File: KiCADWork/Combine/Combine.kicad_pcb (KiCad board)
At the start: 2 copper layers, 100 x 100 mm, 147 parts, among them J1 USB_C_Receptacle, J3 USB_C_Receptacle, J4 Conn_01x10_Socket, J4 Screw_Terminal_01x01, J5 Screw_Terminal_01x02, J6 USB_C_Receptacle, J7 Screw_Terminal_01x01, J8 Screw_Terminal_01x02, P1 USB_C_Plug, P2 USB_C_Plug, SW1 TK-6580B-1, SW2 SW_DIP_x01, SW3 TK-6580B-1, U1 AMS1117-3.3, U2 BQ24073RGT, U3 TPS61023DRLR, U4 SIP32509DT-T1-GE3, U5 USB2422T-I/MJ, U6 SIP32509DT-T1-GE3, U7 MCP73831T-2ACI/OT, U8 XB6096I2SV, U9 NRF52833-QDAA-R7, Y1 X322524MOB4SI, Y2 X161032768KLD2SI, Y3 XL7EL89CKI-111YLC-32M

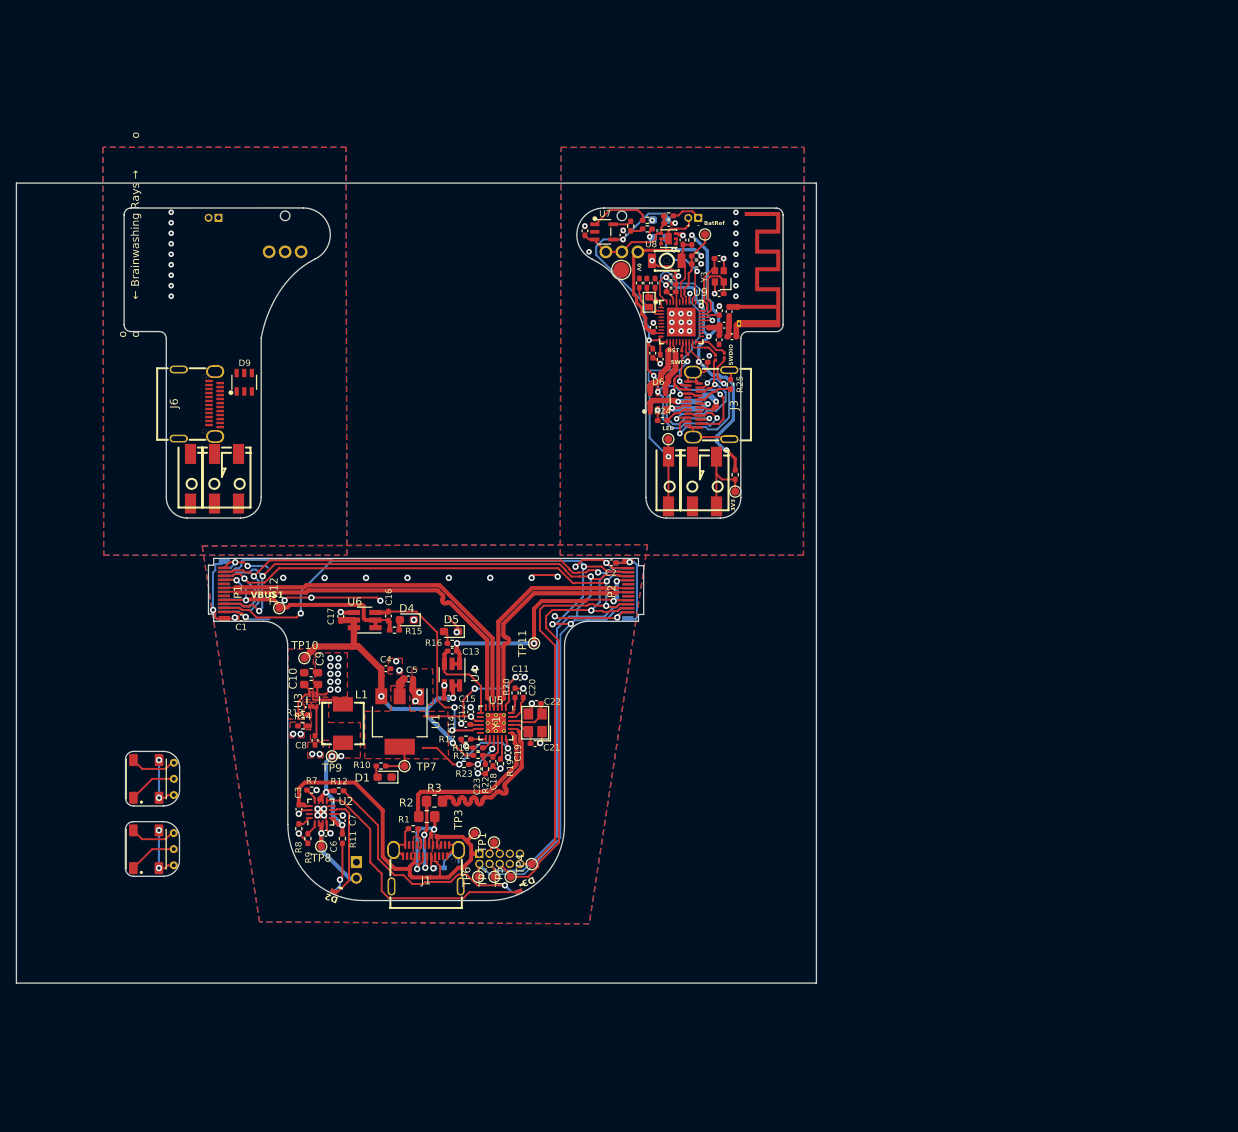
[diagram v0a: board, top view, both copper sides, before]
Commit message: Schem rev 1 pt1
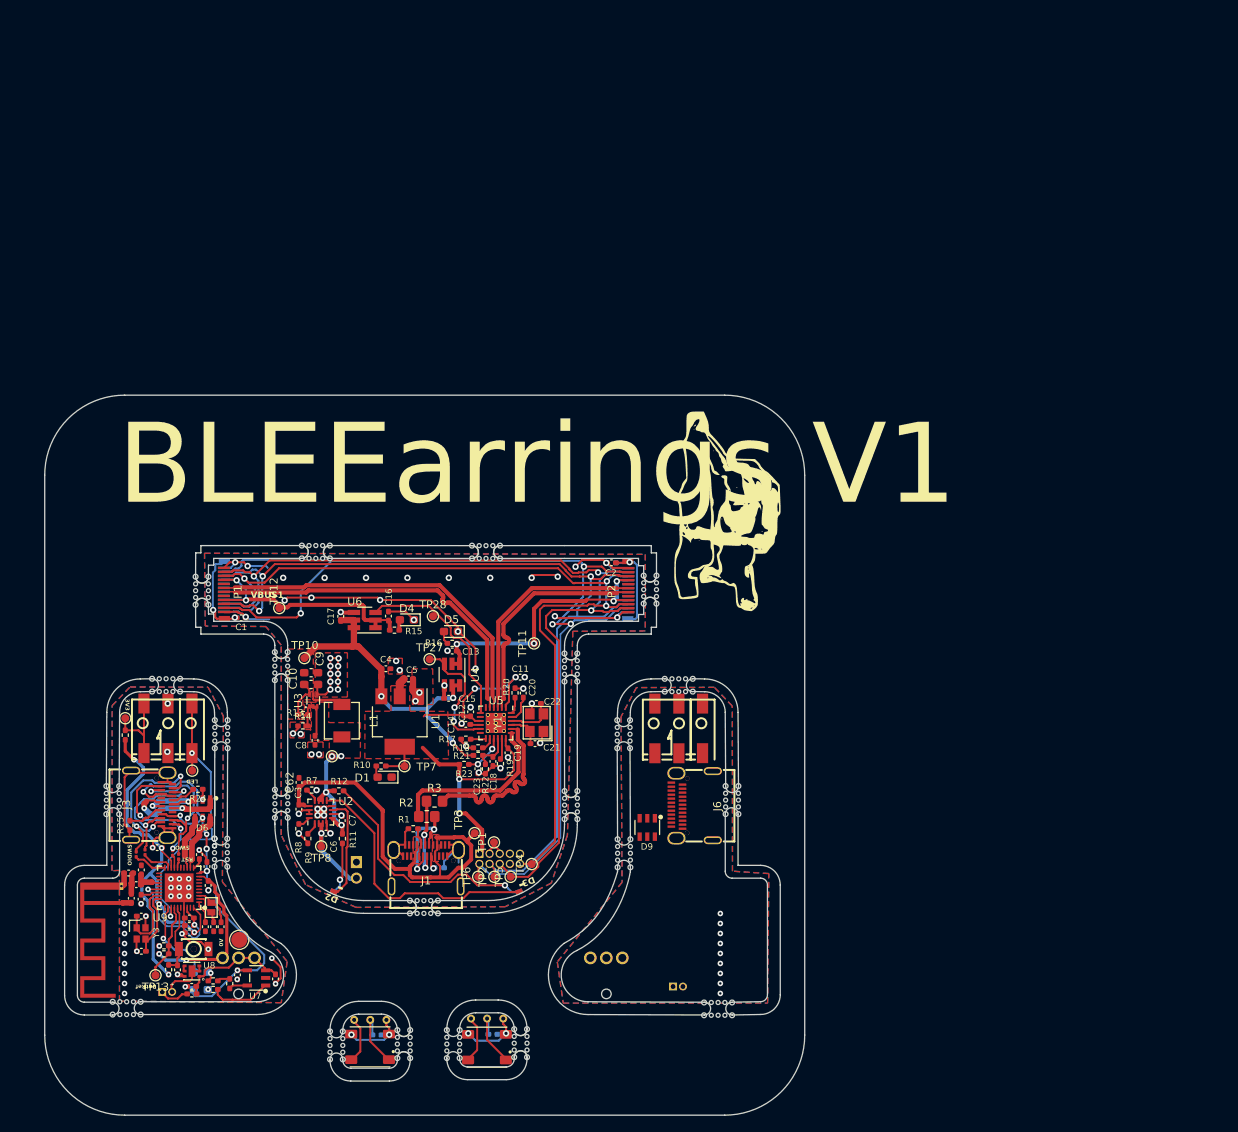
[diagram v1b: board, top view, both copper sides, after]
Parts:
- removed the TP9 at (133.5, 115.2)
- added ?: , , F.Cu at (118.8, 125.5)
- added ?: , , F.Cu at (118.8, 126.4)
- added C62: 10u, Capacitor_SMD:C_0402_1005Metric_Pad0.74x0.62mm_HandSolder, F.Cu at (129.4, 118.5)
- added C63: 100n, Capacitor_SMD:C_0402_1005Metric_Pad0.74x0.62mm_HandSolder, B.Cu at (153.6, 150.0)
- added C64: 100n, Capacitor_SMD:C_0402_1005Metric_Pad0.74x0.62mm_HandSolder, B.Cu at (139.1, 150.0)
- added G***: LOGO, CustomPads:OT2, F.Cu at (182.7, 84.4)
- added REF**: mouse-bit-1.6mm-slot, Panelization:mouse-bit-1.6mm-slot, F.Cu at (127.2, 121.1)
- added REF**: mouse-bit-1.6mm-slot, Panelization:mouse-bit-1.6mm-slot, F.Cu at (163.4, 121.3)
- added REF**: mouse-bit-1.6mm-slot, Panelization:mouse-bit-1.6mm-slot, F.Cu at (157.1, 151.1)
- added REF**: mouse-bit-1.6mm-slot, Panelization:mouse-bit-1.6mm-slot, B.Cu at (181.8, 146.8)
- added REF**: mouse-bit-1.6mm-slot, Panelization:mouse-bit-1.6mm-slot, B.Cu at (112.8, 106.3)
- added REF**: mouse-bit-1.6mm-slot, Panelization:mouse-bit-1.6mm-slot, B.Cu at (134.1, 151.3)
- added REF**: mouse-bit-1.6mm-slot, Panelization:mouse-bit-1.6mm-slot, B.Cu at (107.8, 146.7)
- added REF**: mouse-bit-1.6mm-slot, Panelization:mouse-bit-1.6mm-slot, B.Cu at (106.1, 120.7)
- added REF**: mouse-bit-1.6mm-slot, Panelization:mouse-bit-1.6mm-slot, B.Cu at (183.5, 120.7)
- added REF**: mouse-bit-1.6mm-slot, Panelization:mouse-bit-1.6mm-slot, B.Cu at (119.7, 112.4)
- added REF**: mouse-bit-1.6mm-slot, Panelization:mouse-bit-1.6mm-slot, B.Cu at (119.6, 127.3)
- added REF**: mouse-bit-1.6mm-slot, Panelization:mouse-bit-1.6mm-slot, F.Cu at (127.2, 103.9)
- added REF**: mouse-bit-1.6mm-slot, Panelization:mouse-bit-1.6mm-slot, B.Cu at (148.7, 151.2)
- added REF**: mouse-bit-1.6mm-slot, Panelization:mouse-bit-1.6mm-slot, B.Cu at (170.0, 127.3)
- added REF**: mouse-bit-1.6mm-slot, Panelization:mouse-bit-1.6mm-slot, B.Cu at (170.0, 112.4)
- added REF**: mouse-bit-1.6mm-slot, Panelization:mouse-bit-1.6mm-slot, B.Cu at (176.8, 106.3)
- added REF**: mouse-bit-1.6mm-slot, Panelization:mouse-bit-1.6mm-slot, F.Cu at (117.2, 94.5)
- added REF**: mouse-bit-1.6mm-slot, Panelization:mouse-bit-1.6mm-slot, F.Cu at (163.4, 104.1)
- added REF**: mouse-bit-1.6mm-slot, Panelization:mouse-bit-1.6mm-slot, F.Cu at (145.0, 134.1)
- added REF**: mouse-bit-1.6mm-slot, Panelization:mouse-bit-1.6mm-slot, F.Cu at (142.5, 151.2)
- added REF**: mouse-bit-1.6mm-slot, Panelization:mouse-bit-1.6mm-slot, F.Cu at (173.3, 94.4)
- added REF**: mouse-bit-1.6mm-slot, Panelization:mouse-bit-1.6mm-slot, F.Cu at (152.8, 89.7)
- added REF**: mouse-bit-1.6mm-slot, Panelization:mouse-bit-1.6mm-slot, F.Cu at (131.5, 89.7)
- added TP13: TestPoint, TestPoint:TestPoint_Pad_D1.0mm, F.Cu at (111.4, 142.6)
- added TP27: TestPoint, TestPoint:TestPoint_Pad_D1.0mm, F.Cu at (145.7, 103.1)
- added TP28: TestPoint, TestPoint:TestPoint_Pad_D1.0mm, F.Cu at (146.1, 97.7)
- L1: footprint easyeda2kicad:IND-SMD_L5.2-W5.2_YSPI0530 -> easyeda2kicad:IND-SMD_L4.4-W4.2
- moved BT2 117.0 mm to (112.9, 144.7), turned to 0 degrees
- moved R28 114.1 mm to (116.0, 144.9), turned to 0 degrees
- moved C40 112.8 mm to (109.7, 139.6), turned to 0 degrees
- moved C25 112.5 mm to (116.0, 144.0), turned to 180 degrees
- moved BT3 112.3 mm to (176.8, 144.0), turned to 0 degrees
- moved R37 112.2 mm to (113.1, 141.9), turned to -90 degrees
- moved D7 112.0 mm to (117.1, 144.4), turned to 180 degrees
- moved C41 111.0 mm to (114.2, 141.9), turned to 90 degrees
- moved R26 110.4 mm to (118.6, 144.4), turned to 0 degrees
- moved R34 109.7 mm to (112.5, 139.9), turned to 180 degrees
- moved Y3 109.4 mm to (109.6, 137.4), turned to -90 degrees
- moved U8 109.2 mm to (116.0, 142.1), turned to 90 degrees
- moved R29 108.5 mm to (118.6, 143.3), turned to 180 degrees
- moved D8 108.3 mm to (117.1, 142.2), turned to 180 degrees
- moved R35 108.2 mm to (112.5, 138.9), turned to 0 degrees
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- renumbered J4 to J2, TP24 to TP21, TP25 to TP22
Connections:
- ANT1 pad 1: (no net) -> Net-(ANT1-FP)
- ANT1 pad 2: (no net) -> GND
- BT1 pad 1: (no net) -> /Dock/ExtraBattery/VBAT
- BT1 pad 2: (no net) -> GND
- BT2 pad 1: (no net) -> Net-(BT2-+)
- BT2 pad 2: (no net) -> Net-(BT2--)
- BT3 pad 1: (no net) -> Net-(BT3-+)
- BT3 pad 2: (no net) -> Net-(BT3--)
- C1 pad 1: (no net) -> GND
- C1 pad 2: (no net) -> Net-(P1-SHIELD)
- C10 pad 1: (no net) -> /Dock/DeviceSelect/Vsys
- C10 pad 2: (no net) -> GND
- C11 pad 1: (no net) -> GND
- C11 pad 2: (no net) -> +3V3
- C12 pad 1: (no net) -> GND
- C12 pad 2: (no net) -> +3V3
- C13 pad 1: (no net) -> GND
- C13 pad 2: (no net) -> /Dock/DeviceSelect/VBUS1
- C14 pad 1: (no net) -> GND
- C14 pad 2: (no net) -> Net-(U5-CRFILT)
- C15 pad 1: (no net) -> GND
- C15 pad 2: (no net) -> /Dock/DeviceSelect/Vsys
- C16 pad 1: (no net) -> GND
- C16 pad 2: (no net) -> /Dock/DeviceSelect/VBUS2
- C17 pad 1: (no net) -> GND
- C17 pad 2: (no net) -> /Dock/DeviceSelect/Vsys
- C18 pad 1: (no net) -> GND
- C18 pad 2: (no net) -> Net-(U5-VBUS_DET)
- C19 pad 1: (no net) -> GND
- C19 pad 2: (no net) -> +3V3
- C2 pad 1: (no net) -> GND
- C2 pad 2: (no net) -> Net-(P2-SHIELD)
- C20 pad 1: (no net) -> GND
- C20 pad 2: (no net) -> Net-(U5-PLLFILT)
- C21 pad 1: (no net) -> Net-(U5-XTALOUT/(CLKIN_EN))
- C21 pad 2: (no net) -> GND
- C22 pad 1: (no net) -> GND
- C22 pad 2: (no net) -> Net-(U5-XTALIN/CLKIN)
- C23 pad 1: (no net) -> GND
- C23 pad 2: (no net) -> RESET
- C24 pad 1: (no net) -> /Earring1/Power/VBAT
- C24 pad 2: (no net) -> GND
- C25 pad 1: (no net) -> /Earring1/Power/VBAT
- C25 pad 2: (no net) -> GND
- C26 pad 1: (no net) -> /Earring1/DSP/VBUS
- C26 pad 2: (no net) -> GND
- C27 pad 1: (no net) -> GND
- C27 pad 2: (no net) -> Net-(U9-P0.00_XL1)
- C28 pad 1: (no net) -> GND
- C28 pad 2: (no net) -> +BATT
- C29 pad 1: (no net) -> GND
- C29 pad 2: (no net) -> /Earring1/DSP/VBUS
- C3 pad 1: (no net) -> /Dock/ExtraBattery/VBUS
- C3 pad 2: (no net) -> GND
- C30 pad 1: (no net) -> +3V3
- C30 pad 2: (no net) -> GND
- C31 pad 1: (no net) -> GND
- C31 pad 2: (no net) -> Net-(U9-DECUSB)
- C32 pad 1: (no net) -> GND
- C32 pad 2: (no net) -> Net-(U9-P0.01_XL2)
- C33 pad 1: (no net) -> GND
- C33 pad 2: (no net) -> Net-(U9-DEC1)
- C34 pad 1: (no net) -> GND
- C34 pad 2: (no net) -> +3V3
- C35 pad 1: (no net) -> Net-(U9-ANT)
- C35 pad 2: (no net) -> GND
- C36 pad 1: (no net) -> Net-(U9-DEC3)
- C36 pad 2: (no net) -> GND
- C37 pad 1: (no net) -> Net-(C37-Pad1)
- C37 pad 2: (no net) -> GND
- C38 pad 1: (no net) -> DEC6
- C38 pad 2: (no net) -> GND
- C39 pad 1: (no net) -> DEC6
- C39 pad 2: (no net) -> GND
- C4 pad 1: (no net) -> /Dock/DeviceSelect/Vsys
- C4 pad 2: (no net) -> GND
- C40 pad 1: (no net) -> GND
- C40 pad 2: (no net) -> Net-(U9-XC2)
- C41 pad 1: (no net) -> GND
- C41 pad 2: (no net) -> Pair
- C42 pad 1: (no net) -> GND
- C42 pad 2: (no net) -> Net-(U9-XC1)
- C5 pad 1: (no net) -> +3V3
- C5 pad 2: (no net) -> GND
- C6 pad 1: (no net) -> /Dock/ExtraBattery/VBAT
- C6 pad 2: (no net) -> GND
- C7 pad 1: (no net) -> /Dock/ExtraBattery/3.7Out
- C7 pad 2: (no net) -> GND
- C8 pad 1: (no net) -> /Dock/ExtraBattery/3.7Out
- C8 pad 2: (no net) -> GND
- C9 pad 1: (no net) -> /Dock/DeviceSelect/Vsys
- C9 pad 2: (no net) -> GND
- D1 pad 1: (no net) -> GND
- D1 pad 2: (no net) -> Net-(D1-A)
- D12 pad 1: (no net) -> Net-(D12-VDD)
- D12 pad 2: (no net) -> Net-(D12-DOUT)
- D12 pad 3: (no net) -> Net-(D12-DOUT)
- D12 pad 4: (no net) -> Net-(D12-DIN)
- D13 pad 1: (no net) -> Net-(D13-VDD)
- D13 pad 2: (no net) -> Net-(D13-DOUT)
- D13 pad 3: (no net) -> Net-(D13-DOUT)
- D13 pad 4: (no net) -> Net-(D13-DIN)
- D2 pad 1: (no net) -> Net-(D2-K)
- D2 pad 2: (no net) -> Net-(D2-A)
- D3 pad 1: (no net) -> Net-(D3-K)
- D3 pad 2: (no net) -> Net-(D3-A)
- D4 pad 1: (no net) -> GND
- D4 pad 2: (no net) -> Net-(D4-A)
- D5 pad 1: (no net) -> GND
- D5 pad 2: (no net) -> Net-(D5-A)
- D6 pad 1: (no net) -> Net-(D6-I/O1-Pad1)
- D6 pad 2: (no net) -> GND
- D6 pad 3: (no net) -> Net-(D6-I/O2-Pad3)
- D6 pad 4: (no net) -> D+
- D6 pad 5: (no net) -> /Earring1/DSP/VBUS
- D6 pad 6: (no net) -> D-
- D7 pad 1: (no net) -> Net-(D7-K)
- D7 pad 2: (no net) -> /Earring1/DSP/VBUS
- D8 pad 1: (no net) -> Net-(D8-K)
- D8 pad 2: (no net) -> LED_A
- D9 pad 1: (no net) -> Net-(D9-I/O1-Pad1)
- D9 pad 2: (no net) -> GND
- D9 pad 3: (no net) -> Net-(D9-I/O2-Pad3)
- D9 pad 4: (no net) -> D+
- D9 pad 5: (no net) -> /Earring2/DSP/VBUS
- D9 pad 6: (no net) -> D-
- J1 pad A1: (no net) -> GND
- J1 pad A10: (no net) -> unconnected-(J1-RX2--PadA10)
- J1 pad A11: (no net) -> unconnected-(J1-RX2+-PadA11)
- J1 pad A2: (no net) -> unconnected-(J1-TX1+-PadA2)
- J1 pad A3: (no net) -> unconnected-(J1-TX1--PadA3)
- J1 pad A4: (no net) -> /Dock/ExtraBattery/VBUS
- J1 pad A5: (no net) -> Net-(J1-CC1)
- J1 pad A6: (no net) -> Net-(J1-D+-PadA6)
- J1 pad A7: (no net) -> Net-(J1-D--PadA7)
- J1 pad A8: (no net) -> unconnected-(J1-SBU1-PadA8)
- J1 pad B10: (no net) -> unconnected-(J1-RX1--PadB10)
- J1 pad B11: (no net) -> unconnected-(J1-RX1+-PadB11)
- J1 pad B2: (no net) -> unconnected-(J1-TX2+-PadB2)
- J1 pad B3: (no net) -> unconnected-(J1-TX2--PadB3)
- J1 pad B5: (no net) -> Net-(J1-CC2)
- J1 pad B6: (no net) -> Net-(J1-D+-PadA6)
- J1 pad B7: (no net) -> Net-(J1-D--PadA7)
- J1 pad B8: (no net) -> unconnected-(J1-SBU2-PadB8)
- J1 pad S1: (no net) -> GND
- J2 pad 1: (no net) -> +3V3
- J2 pad 10: (no net) -> nRESET
- J2 pad 2: (no net) -> SWDIO
- J2 pad 3: (no net) -> GND
- J2 pad 4: (no net) -> SWCLK
- J2 pad 5: (no net) -> GND
- J2 pad 6: (no net) -> SWO
- J2 pad 7: (no net) -> unconnected-(J2-Pin_7-Pad7)
- J2 pad 8: (no net) -> unconnected-(J2-Pin_8-Pad8)
- J2 pad 9: (no net) -> unconnected-(J2-Pin_9-Pad9)
- J3 pad A1: (no net) -> GND
- J3 pad A10: (no net) -> /Earring1/DSP/nReset
- J3 pad A11: (no net) -> SWO_L
- J3 pad A2: (no net) -> SWDIO_L
- J3 pad A3: (no net) -> SWDCLK_L
- J3 pad A4: (no net) -> /Earring1/DSP/VBUS
- J3 pad A5: (no net) -> Net-(J3-CC1)
- J3 pad A6: (no net) -> Net-(D6-I/O2-Pad3)
- J3 pad A7: (no net) -> Net-(D6-I/O1-Pad1)
- J3 pad A8: (no net) -> unconnected-(J3-SBU1-PadA8)
- J3 pad B10: (no net) -> /Earring1/DSP/nReset
- J3 pad B11: (no net) -> SWO_L
- J3 pad B2: (no net) -> SWDIO_L
- J3 pad B3: (no net) -> SWDCLK_L
- J3 pad B5: (no net) -> Net-(J3-CC2)
- J3 pad B6: (no net) -> Net-(D6-I/O2-Pad3)
- J3 pad B7: (no net) -> Net-(D6-I/O1-Pad1)
- J3 pad B8: (no net) -> unconnected-(J3-SBU2-PadB8)
- J3 pad S1: (no net) -> GND
- J4 pad 1: (no net) -> NEO_LED
- J5 pad 1: (no net) -> Net-(J5-Pin_1)
- J5 pad 2: (no net) -> GND
- J6 pad A1: (no net) -> GND
- J6 pad A10: (no net) -> /Earring2/DSP/nReset
- J6 pad A11: (no net) -> SWO_L
- J6 pad A2: (no net) -> SWDIO_L
- J6 pad A3: (no net) -> SWDCLK_L
- J6 pad A4: (no net) -> /Earring2/DSP/VBUS
- J6 pad A5: (no net) -> Net-(J6-CC1)
- J6 pad A6: (no net) -> Net-(D9-I/O2-Pad3)
- J6 pad A7: (no net) -> Net-(D9-I/O1-Pad1)
- J6 pad A8: (no net) -> unconnected-(J6-SBU1-PadA8)
- J6 pad B10: (no net) -> /Earring2/DSP/nReset
- J6 pad B11: (no net) -> SWO_L
- J6 pad B2: (no net) -> SWDIO_L
- J6 pad B3: (no net) -> SWDCLK_L
- J6 pad B5: (no net) -> Net-(J6-CC2)
- J6 pad B6: (no net) -> Net-(D9-I/O2-Pad3)
- J6 pad B7: (no net) -> Net-(D9-I/O1-Pad1)
- J6 pad B8: (no net) -> unconnected-(J6-SBU2-PadB8)
- J6 pad S1: (no net) -> GND
- J7 pad 1: (no net) -> NEO_LED
- J8 pad 1: (no net) -> Net-(J8-Pin_1)
- J8 pad 2: (no net) -> GND
- L1 pad 1: (no net) -> /Dock/ExtraBattery/3.7Out
- L1 pad 2: (no net) -> Net-(U3-SW)
- L2 pad 1: (no net) -> Net-(U9-ANT)
- L2 pad 2: (no net) -> Net-(C37-Pad1)
- L3 pad 1: (no net) -> Net-(C37-Pad1)
- L3 pad 2: (no net) -> Net-(ANT1-FP)
- P1 pad A1: (no net) -> GND
- P1 pad A10: (no net) -> nRESET
- P1 pad A11: (no net) -> SWO
- P1 pad A2: (no net) -> SWDIO
- P1 pad A3: (no net) -> SWCLK
- P1 pad A4: (no net) -> /Dock/DeviceSelect/VBUS2
- P1 pad A5: (no net) -> unconnected-(P1-CC-PadA5)
- P1 pad A6: (no net) -> /Dock/DeviceSelect/D2+
- P1 pad A7: (no net) -> /Dock/DeviceSelect/D2-
- P1 pad A8: (no net) -> unconnected-(P1-SBU1-PadA8)
- P1 pad A9: (no net) -> /Dock/DeviceSelect/VBUS2
- P1 pad B10: (no net) -> nRESET
- P1 pad B11: (no net) -> SWO
- P1 pad B2: (no net) -> SWDIO
- P1 pad B3: (no net) -> SWCLK
- P1 pad B4: (no net) -> /Dock/DeviceSelect/VBUS2
- P1 pad B5: (no net) -> unconnected-(P1-VCONN-PadB5)
- P1 pad B8: (no net) -> unconnected-(P1-SBU2-PadB8)
- P1 pad B9: (no net) -> /Dock/DeviceSelect/VBUS2
- P1 pad S1: (no net) -> Net-(P1-SHIELD)
- P2 pad A1: (no net) -> GND
- P2 pad A10: (no net) -> nRESET
- P2 pad A11: (no net) -> SWO
- P2 pad A2: (no net) -> SWDIO
- P2 pad A3: (no net) -> SWCLK
- P2 pad A4: (no net) -> /Dock/DeviceSelect/VBUS1
- P2 pad A5: (no net) -> unconnected-(P2-CC-PadA5)
- P2 pad A6: (no net) -> /Dock/DeviceSelect/D1+
- P2 pad A7: (no net) -> /Dock/DeviceSelect/D1-
- P2 pad A8: (no net) -> unconnected-(P2-SBU1-PadA8)
- P2 pad A9: (no net) -> /Dock/DeviceSelect/VBUS1
- P2 pad B10: (no net) -> nRESET
- P2 pad B11: (no net) -> SWO
- P2 pad B2: (no net) -> SWDIO
- P2 pad B3: (no net) -> SWCLK
- P2 pad B4: (no net) -> /Dock/DeviceSelect/VBUS1
- P2 pad B5: (no net) -> unconnected-(P2-VCONN-PadB5)
- P2 pad B8: (no net) -> unconnected-(P2-SBU2-PadB8)
- P2 pad B9: (no net) -> /Dock/DeviceSelect/VBUS1
- P2 pad S1: (no net) -> Net-(P2-SHIELD)
- R1 pad 1: (no net) -> GND
- R1 pad 2: (no net) -> Net-(J1-CC1)
- R10 pad 1: (no net) -> Net-(D1-A)
- R10 pad 2: (no net) -> +3V3
- R11 pad 1: (no net) -> Net-(D2-A)
- R11 pad 2: (no net) -> /Dock/ExtraBattery/3.7Out
- R12 pad 1: (no net) -> Net-(D3-A)
- R12 pad 2: (no net) -> /Dock/ExtraBattery/3.7Out
- R13 pad 1: (no net) -> /Dock/ExtraBattery/FB
- R13 pad 2: (no net) -> /Dock/DeviceSelect/Vsys
- R14 pad 1: (no net) -> GND
- R14 pad 2: (no net) -> /Dock/ExtraBattery/FB
- R15 pad 1: (no net) -> /Dock/DeviceSelect/VBUS2
- R15 pad 2: (no net) -> Net-(D4-A)
- R16 pad 1: (no net) -> /Dock/DeviceSelect/VBUS1
- R16 pad 2: (no net) -> Net-(D5-A)
- R17 pad 1: (no net) -> GND
- R17 pad 2: (no net) -> Net-(U5-SMBDATA/NON_REM1)
- R18 pad 1: (no net) -> GND
- R18 pad 2: (no net) -> Net-(U5-SMBCLK/CFG_SEL0)
- R19 pad 1: (no net) -> GND
- R19 pad 2: (no net) -> Net-(U5-SUSP_IND/LOCAL_PWR/(NON_REM0))
- R2 pad 1: (no net) -> Net-(J1-D--PadA7)
- R2 pad 2: (no net) -> /Dock/DeviceSelect/D-
- R20 pad 1: (no net) -> GND
- R20 pad 2: (no net) -> Net-(U5-RBIAS)
- R21 pad 1: (no net) -> Net-(U5-VBUS_DET)
- R21 pad 2: (no net) -> /Dock/DeviceSelect/Vsys
- R22 pad 1: (no net) -> GND
- R22 pad 2: (no net) -> Net-(U5-VBUS_DET)
- R23 pad 1: (no net) -> RESET
- R23 pad 2: (no net) -> +3V3
- R24 pad 1: (no net) -> GND
- R24 pad 2: (no net) -> Net-(J3-CC1)
- R25 pad 1: (no net) -> GND
- R25 pad 2: (no net) -> Net-(J3-CC2)
- R26 pad 1: (no net) -> Net-(D7-K)
- R26 pad 2: (no net) -> Net-(U7-STAT)
- R27 pad 1: (no net) -> Net-(U7-PROG)
- R27 pad 2: (no net) -> GND
- R28 pad 1: (no net) -> Net-(BT2-+)
- R28 pad 2: (no net) -> /Earring1/Power/VBAT
- R29 pad 1: (no net) -> GND
- R29 pad 2: (no net) -> Net-(D8-K)
- R3 pad 1: (no net) -> /Dock/DeviceSelect/D+
- R3 pad 2: (no net) -> Net-(J1-D+-PadA6)
- R30 pad 1: (no net) -> Net-(U9-P0.20)
- R30 pad 2: (no net) -> SWO_L
- R31 pad 1: (no net) -> Net-(U9-SWDCLK)
- R31 pad 2: (no net) -> SWDIO_L
- R32 pad 1: (no net) -> /Earring1/DSP/nReset
- R32 pad 2: (no net) -> Net-(U9-P0.18_nRESET)
- R33 pad 1: (no net) -> SWDCLK_L
- R33 pad 2: (no net) -> Net-(U9-SWDIO)
- R34 pad 1: (no net) -> BatRef
- R34 pad 2: (no net) -> +BATT
- R35 pad 1: (no net) -> GND
- R35 pad 2: (no net) -> BatRef
- R36 pad 1: (no net) -> Net-(J5-Pin_1)
- R36 pad 2: (no net) -> +3V3
- R37 pad 1: (no net) -> Pair
- R37 pad 2: (no net) -> +3V3
- R4 pad 1: (no net) -> GND
- R4 pad 2: (no net) -> Net-(J1-CC2)
- R5 pad 1: (no net) -> Net-(P1-SHIELD)
- R5 pad 2: (no net) -> GND
- R6 pad 1: (no net) -> Net-(P2-SHIELD)
- R6 pad 2: (no net) -> GND
- R7 pad 1: (no net) -> Net-(U2-ILIM)
- R7 pad 2: (no net) -> GND
- R8 pad 1: (no net) -> Net-(U2-ISET)
- R8 pad 2: (no net) -> GND
- R9 pad 1: (no net) -> GND
- R9 pad 2: (no net) -> Net-(U2-TS)
- SW1 pad 1: (no net) -> /Earring1/Power/VBAT
- SW1 pad 2: (no net) -> /Earring1/Power/VBAT
- SW1 pad 3: (no net) -> +BATT
- SW2 pad 1: (no net) -> Pair
- SW2 pad 2: (no net) -> GND
- SW3 pad 1: (no net) -> /Earring2/Power/VBAT
- SW3 pad 2: (no net) -> /Earring2/Power/VBAT
- SW3 pad 3: (no net) -> +BATT
- TP1 pad 1: (no net) -> GND
- TP10 pad 1: (no net) -> /Dock/DeviceSelect/Vsys
- TP11 pad 1: (no net) -> /Dock/DeviceSelect/VBUS1
- TP12 pad 1: (no net) -> /Dock/DeviceSelect/VBUS2
- TP14 pad 1: (no net) -> NEO_LED
- TP15 pad 1: (no net) -> Net-(J5-Pin_1)
- TP16 pad 1: (no net) -> GND
- TP2 pad 1: (no net) -> SWCLK
- TP21 pad 1: (no net) -> Net-(D12-DIN)
- TP22 pad 1: (no net) -> Net-(D12-VDD)
- TP23 pad 1: (no net) -> Net-(D12-DOUT)
- TP24 pad 1: (no net) -> Net-(D13-DIN)
- TP25 pad 1: (no net) -> Net-(D13-VDD)
- TP26 pad 1: (no net) -> Net-(D13-DOUT)
- TP3 pad 1: (no net) -> /Dock/ExtraBattery/VBUS
- TP4 pad 1: (no net) -> nRESET
- TP5 pad 1: (no net) -> SWO
- TP6 pad 1: (no net) -> SWDIO
- TP7 pad 1: (no net) -> +3V3
- TP8 pad 1: (no net) -> /Dock/ExtraBattery/VBAT
- TP9 pad 1: (no net) -> /Dock/ExtraBattery/3.7Out
- U1 pad 1: (no net) -> GND
- U1 pad 2: (no net) -> +3V3
- U1 pad 3: (no net) -> /Dock/DeviceSelect/Vsys
- U2 pad 1: (no net) -> Net-(U2-TS)
- U2 pad 10: (no net) -> /Dock/ExtraBattery/3.7Out
- U2 pad 11: (no net) -> /Dock/ExtraBattery/3.7Out
- U2 pad 12: (no net) -> Net-(U2-ILIM)
- U2 pad 13: (no net) -> /Dock/ExtraBattery/VBUS
- U2 pad 14: (no net) -> GND
- U2 pad 15: (no net) -> GND
- U2 pad 16: (no net) -> Net-(U2-ISET)
- U2 pad 17: (no net) -> GND
- U2 pad 2: (no net) -> /Dock/ExtraBattery/VBAT
- U2 pad 3: (no net) -> /Dock/ExtraBattery/VBAT
- U2 pad 4: (no net) -> GND
- U2 pad 5: (no net) -> /Dock/ExtraBattery/3.7Out
- U2 pad 6: (no net) -> GND
- U2 pad 7: (no net) -> Net-(D2-K)
- U2 pad 8: (no net) -> GND
- U2 pad 9: (no net) -> Net-(D3-K)
- U3 pad 1: (no net) -> /Dock/ExtraBattery/FB
- U3 pad 2: (no net) -> /Dock/ExtraBattery/3.7Out
- U3 pad 3: (no net) -> /Dock/ExtraBattery/3.7Out
- U3 pad 4: (no net) -> GND
- U3 pad 5: (no net) -> Net-(U3-SW)
- U3 pad 6: (no net) -> /Dock/DeviceSelect/Vsys
- U4 pad 1: (no net) -> /Dock/DeviceSelect/VBUS1
- U4 pad 2: (no net) -> /Dock/DeviceSelect/VBUS1
- U4 pad 3: (no net) -> PWREN1
- U4 pad 4: (no net) -> GND
- U4 pad 5: (no net) -> /Dock/DeviceSelect/Vsys
- U4 pad 6: (no net) -> /Dock/DeviceSelect/Vsys
- U5 pad 1: (no net) -> +3V3
- U5 pad 10: (no net) -> Net-(U5-CRFILT)
- U5 pad 11: (no net) -> PWREN1
- U5 pad 12: (no net) -> unconnected-(U5-OCS2_N-Pad12)
- U5 pad 13: (no net) -> Net-(U5-SMBDATA/NON_REM1)
- U5 pad 14: (no net) -> Net-(U5-SMBCLK/CFG_SEL0)
- U5 pad 15: (no net) -> RESET
- U5 pad 16: (no net) -> Net-(U5-VBUS_DET)
- U5 pad 17: (no net) -> Net-(U5-SUSP_IND/LOCAL_PWR/(NON_REM0))
- U5 pad 18: (no net) -> +3V3
- U5 pad 19: (no net) -> /Dock/DeviceSelect/D-
- U5 pad 2: (no net) -> /Dock/DeviceSelect/D1-
- U5 pad 20: (no net) -> /Dock/DeviceSelect/D+
- U5 pad 21: (no net) -> Net-(U5-XTALOUT/(CLKIN_EN))
- U5 pad 22: (no net) -> Net-(U5-XTALIN/CLKIN)
- U5 pad 23: (no net) -> Net-(U5-PLLFILT)
- U5 pad 24: (no net) -> Net-(U5-RBIAS)
- U5 pad 25: (no net) -> GND
- U5 pad 3: (no net) -> /Dock/DeviceSelect/D1+
- U5 pad 4: (no net) -> /Dock/DeviceSelect/D2-
- U5 pad 5: (no net) -> /Dock/DeviceSelect/D2+
- U5 pad 6: (no net) -> unconnected-(U5-NC-Pad6)
- U5 pad 7: (no net) -> PWREN2
- U5 pad 8: (no net) -> unconnected-(U5-OCS1_N-Pad8)
- U5 pad 9: (no net) -> +3V3
- U6 pad 1: (no net) -> /Dock/DeviceSelect/VBUS2
- U6 pad 2: (no net) -> /Dock/DeviceSelect/VBUS2
- U6 pad 3: (no net) -> PWREN2
- U6 pad 4: (no net) -> GND
- U6 pad 5: (no net) -> /Dock/DeviceSelect/Vsys
- U6 pad 6: (no net) -> /Dock/DeviceSelect/Vsys
- U7 pad 1: (no net) -> Net-(U7-STAT)
- U7 pad 2: (no net) -> GND
- U7 pad 3: (no net) -> /Earring1/Power/VBAT
- U7 pad 4: (no net) -> /Earring1/DSP/VBUS
- U7 pad 5: (no net) -> Net-(U7-PROG)
- U8 pad 1: (no net) -> /Earring1/Power/VBAT
- U8 pad 2: (no net) -> Net-(BT2--)
- U8 pad 3: (no net) -> Net-(BT2--)
- U8 pad 4: (no net) -> GND
- U8 pad 5: (no net) -> GND
- U8 pad 6: (no net) -> GND
- U8 pad 7: (no net) -> Net-(BT2--)
- U9 pad 1: (no net) -> Net-(U9-DEC1)
- U9 pad 10: (no net) -> /Earring1/DSP/VBUS
- U9 pad 11: (no net) -> Net-(U9-DECUSB)
- U9 pad 12: (no net) -> D-
- U9 pad 13: (no net) -> D+
- U9 pad 14: (no net) -> unconnected-(U9-P0.15-Pad14)
- U9 pad 15: (no net) -> unconnected-(U9-P0.17-Pad15)
- U9 pad 16: (no net) -> Net-(U9-P0.18_nRESET)
- U9 pad 17: (no net) -> Net-(U9-P0.20)
- U9 pad 18: (no net) -> +3V3
- U9 pad 19: (no net) -> Net-(U9-SWDIO)
- U9 pad 2: (no net) -> Net-(U9-P0.00_XL1)
- U9 pad 20: (no net) -> Net-(U9-SWDCLK)
- U9 pad 21: (no net) -> unconnected-(U9-DEC5-Pad21)
- U9 pad 22: (no net) -> unconnected-(U9-P0.09_NFC1-Pad22)
- U9 pad 23: (no net) -> unconnected-(U9-P0.10_NFC2-Pad23)
- U9 pad 24: (no net) -> Net-(U9-ANT)
- U9 pad 25: (no net) -> unconnected-(U9-VSS_PA-Pad25)
- U9 pad 26: (no net) -> DEC6
- U9 pad 27: (no net) -> Net-(U9-DEC3)
- U9 pad 28: (no net) -> Net-(U9-XC1)
- U9 pad 29: (no net) -> Net-(U9-XC2)
- U9 pad 3: (no net) -> Net-(U9-P0.01_XL2)
- U9 pad 30: (no net) -> +3V3
- U9 pad 31: (no net) -> unconnected-(U9-P0.03_AIN1-Pad31)
- U9 pad 32: (no net) -> LED_A
- U9 pad 33: (no net) -> NEO_LED
- U9 pad 34: (no net) -> BatRef
- U9 pad 35: (no net) -> Pair
- U9 pad 36: (no net) -> unconnected-(U9-P0.31_AIN7-Pad36)
- U9 pad 37: (no net) -> GND
- U9 pad 38: (no net) -> DEC6
- U9 pad 39: (no net) -> unconnected-(U9-DCC-Pad39)
- U9 pad 4: (no net) -> unconnected-(U9-P0.04_AIN2-Pad4)
- U9 pad 40: (no net) -> +3V3
- U9 pad 41: (no net) -> GND
- U9 pad 5: (no net) -> unconnected-(U9-P0.05_AIN3-Pad5)
- U9 pad 6: (no net) -> unconnected-(U9-P1.09-Pad6)
- U9 pad 7: (no net) -> unconnected-(U9-P0.11-Pad7)
- U9 pad 8: (no net) -> unconnected-(U9-VDD-Pad8)
- U9 pad 9: (no net) -> +BATT
- Y1 pad 1: (no net) -> GND
- Y1 pad 2: (no net) -> Net-(U5-XTALIN/CLKIN)
- Y1 pad 3: (no net) -> GND
- Y1 pad 4: (no net) -> Net-(U5-XTALOUT/(CLKIN_EN))
- Y2 pad 1: (no net) -> Net-(U9-P0.01_XL2)
- Y2 pad 2: (no net) -> Net-(U9-P0.00_XL1)
- Y3 pad 1: (no net) -> Net-(U9-XC1)
- Y3 pad 2: (no net) -> GND
- Y3 pad 3: (no net) -> GND
- Y3 pad 4: (no net) -> Net-(U9-XC2)
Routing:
- net (no net): track 1751.1 -> 0.00 mm, vias 187 -> 0
- net GND: track 0.00 -> 183.1 mm, vias 0 -> 105
- net SWDIO: track 0.00 -> 132.3 mm, vias 0 -> 4
- net SWO: track 0.00 -> 117.6 mm, vias 0 -> 3
- net SWCLK: track 0.00 -> 117.4 mm, vias 0 -> 3
- net +3V3: track 0.00 -> 113.5 mm, vias 0 -> 9
- net nRESET: track 0.00 -> 112.8 mm, vias 0 -> 3
- net /Earring1/DSP/VBUS: track 0.00 -> 56.9 mm, vias 0 -> 7
- net /Dock/ExtraBattery/VBUS: track 0.00 -> 52.8 mm
- net /Dock/DeviceSelect/Vsys: track 0.00 -> 46.2 mm, vias 0 -> 3
- net /Dock/DeviceSelect/D2-: track 0.00 -> 45.2 mm
- net /Dock/DeviceSelect/D2+: track 0.00 -> 45.0 mm
- net /Dock/DeviceSelect/VBUS1: track 0.00 -> 38.3 mm, vias 0 -> 4
- net NEO_LED: track 0.00 -> 36.3 mm, vias 0 -> 2
- net /Dock/DeviceSelect/VBUS2: track 0.00 -> 35.1 mm, vias 0 -> 2
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- added copper zone on F.Cu, net +3V3
- added copper zone on F.Cu, net /Dock/DeviceSelect/Vsys
- added copper zone on F.Cu, net /Dock/ExtraBattery/3.7Out
- added copper zone on F.Cu, net /Dock/ExtraBattery/FB
- added copper zone on B.Cu, net GND
- added copper zone on F.Cu, net GND
- removed copper zone on B.Cu, net (none)
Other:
- board size 100 x 100 mm -> 95 x 90 mm
- board text added: "BLEEarrings V1"
